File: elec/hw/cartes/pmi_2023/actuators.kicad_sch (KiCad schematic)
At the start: 38 parts, among them J1 con_servo, J2 con_servo, J3 con_servo, J4 con_servo, U23 PCA9685PW, U24 SN74LVC1T45DBV, U25 SN74LVC1T45DBV, U26 SN74LVC1T45DBV, U27 SN74LVC1T45DBV

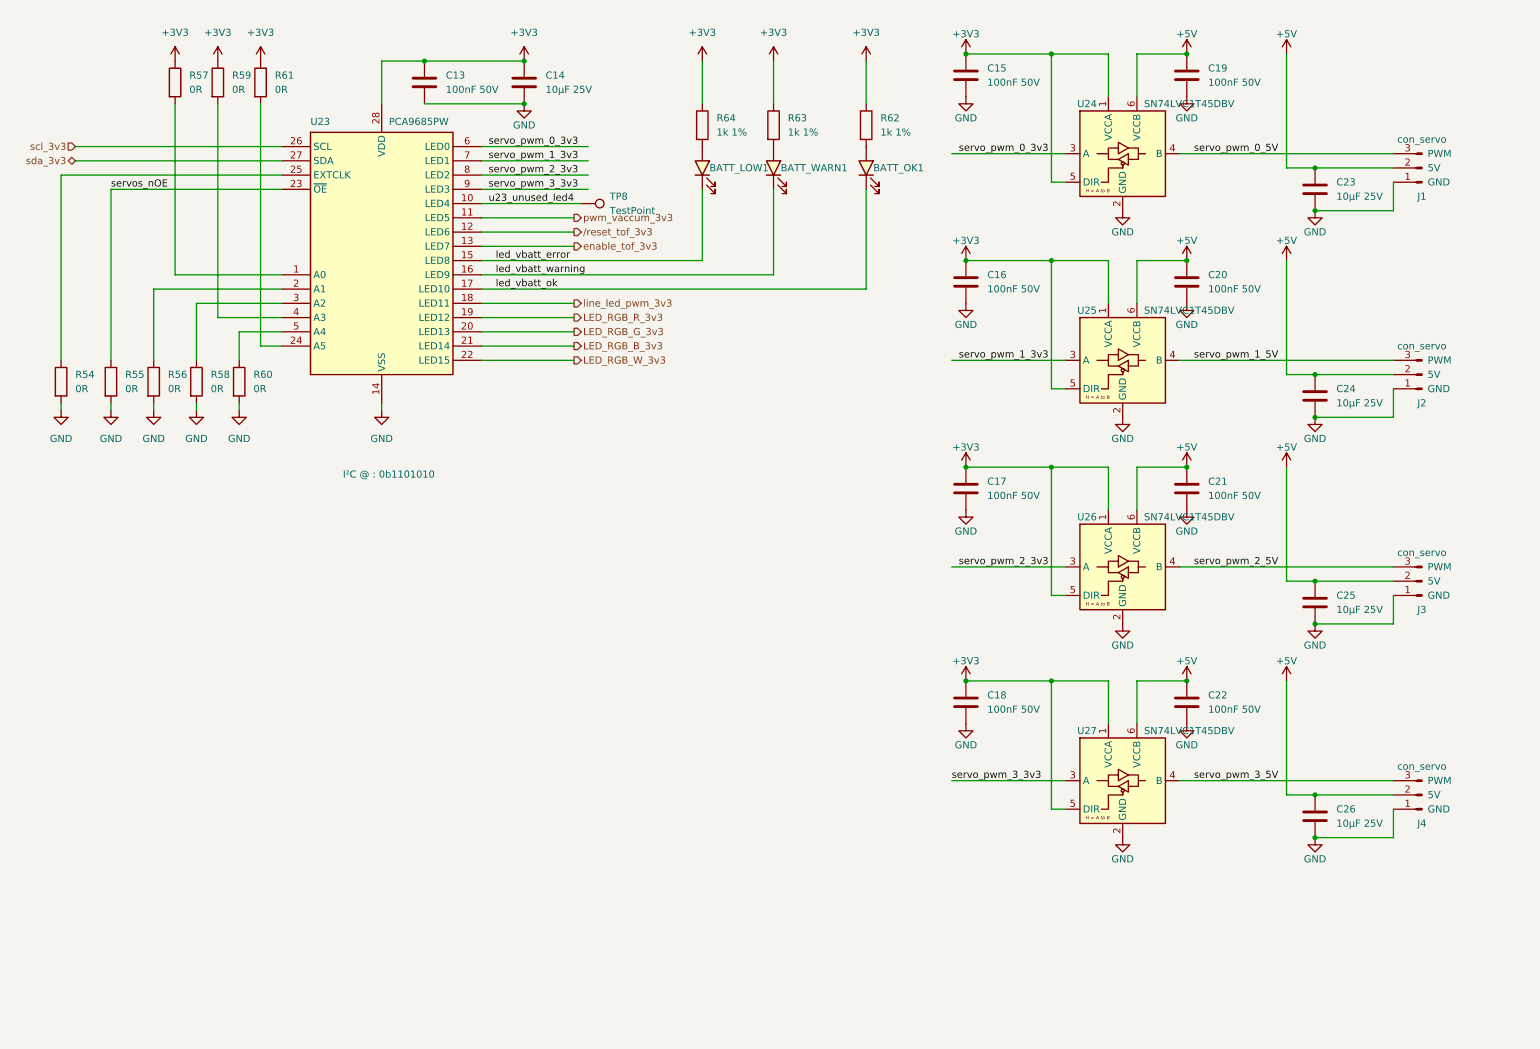
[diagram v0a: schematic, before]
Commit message: wip
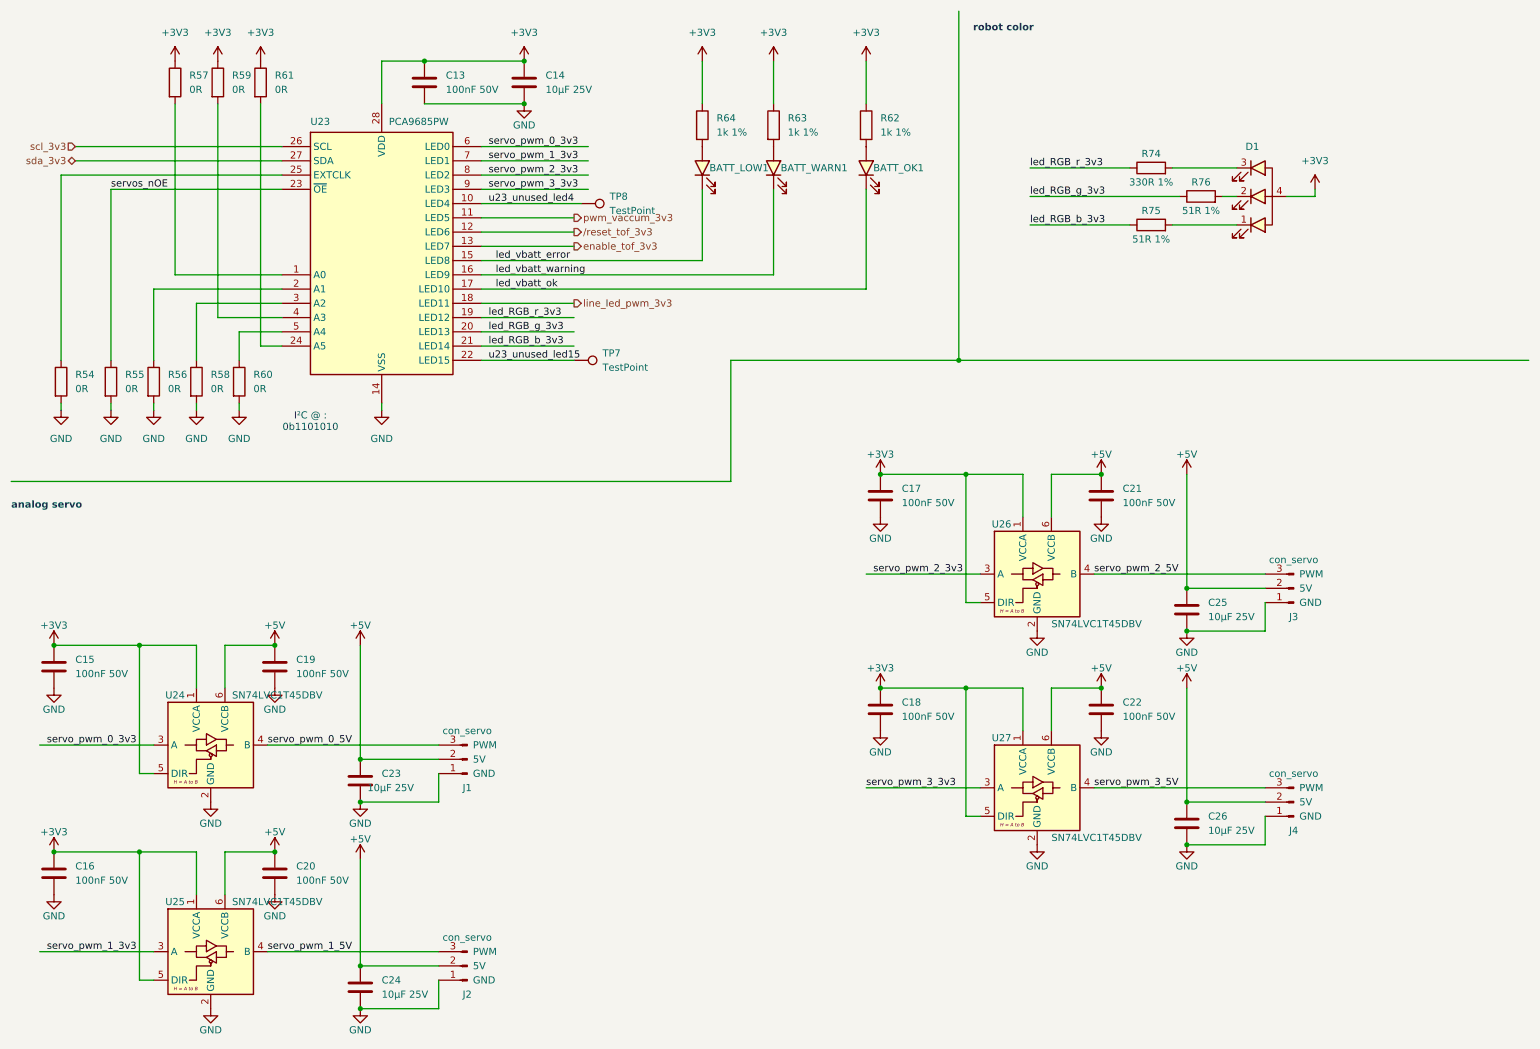
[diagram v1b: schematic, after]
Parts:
- added D1: ~, cocotter_diodes:3528_PLCC-Reverse_mount, symbol cocotter_diodes:IN-P32TRRRGB
- added R74: 330R 1%, cocotter_resistor:r0603_reflow, symbol cocotter_resistors:R_330R_0603_1%
- added R75, R76: 51R 1%, cocotter_resistor:r0603_reflow, symbol cocotter_resistors:R_51R_0603_1%
- added TP7: TestPoint, cocotter_others:testpoint-THT-0.5mm, symbol cocotter_others:TestPoint
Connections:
- net +3V3: now also D1.4 (COM)
- net LED_RGB_B_3v3 renamed led_RGB_b_3v3
- net led_RGB_b_3v3: now also R75.1
- net LED_RGB_G_3v3 renamed led_RGB_g_3v3
- net led_RGB_g_3v3: now also R76.1
- net LED_RGB_R_3v3 renamed led_RGB_r_3v3
- net led_RGB_r_3v3: now also R74.1
- net LED_RGB_W_3v3 renamed u23_unused_led15
- net u23_unused_led15: now also TP7.1
- new net: D1.1 (C_BLUE), R75.2
- new net: D1.2 (C_GREEN), R76.2
- new net: D1.3 (C_RED), R74.2
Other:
- note added: "analog servo"
- note added: "robot color"
- moved on the sheet: C15, C16, C17, C18, C19, C20, C21, C22, C23, C24, C25, C26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
